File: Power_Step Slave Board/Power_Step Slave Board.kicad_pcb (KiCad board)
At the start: 2 copper layers, 69.4 x 49.1 mm, 23 parts, among them P1 CONN_01X04, P10 CONN_01X04, P11 CONN_01X02, P12 CONN_01X04, P13 CONN_01X04, P2 CONN_01X04, P3 CONN_01X02, P4 CONN_01X02, P5 CONN_01X04, P6 CONN_01X02, P7 CONN_01X04, P8 CONN_01X02, P9 CONN_01X04

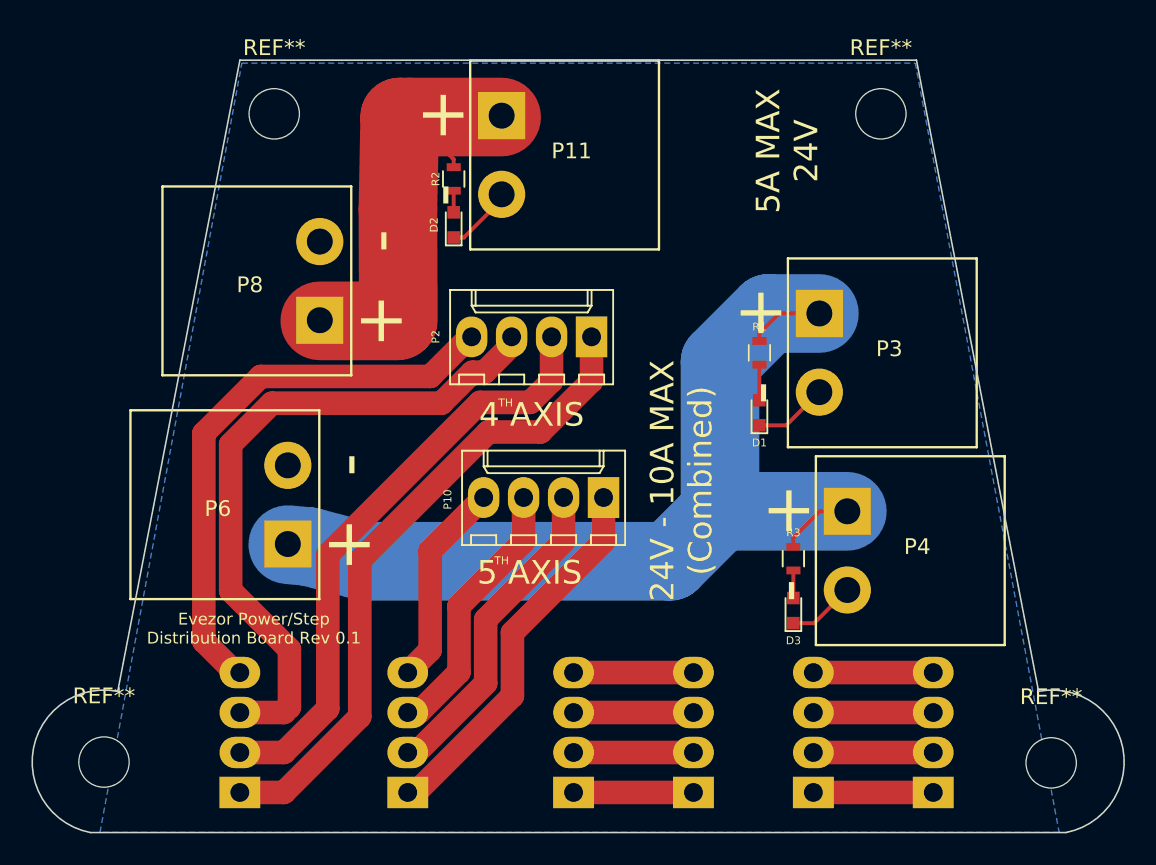
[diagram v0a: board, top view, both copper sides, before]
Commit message: more fixes
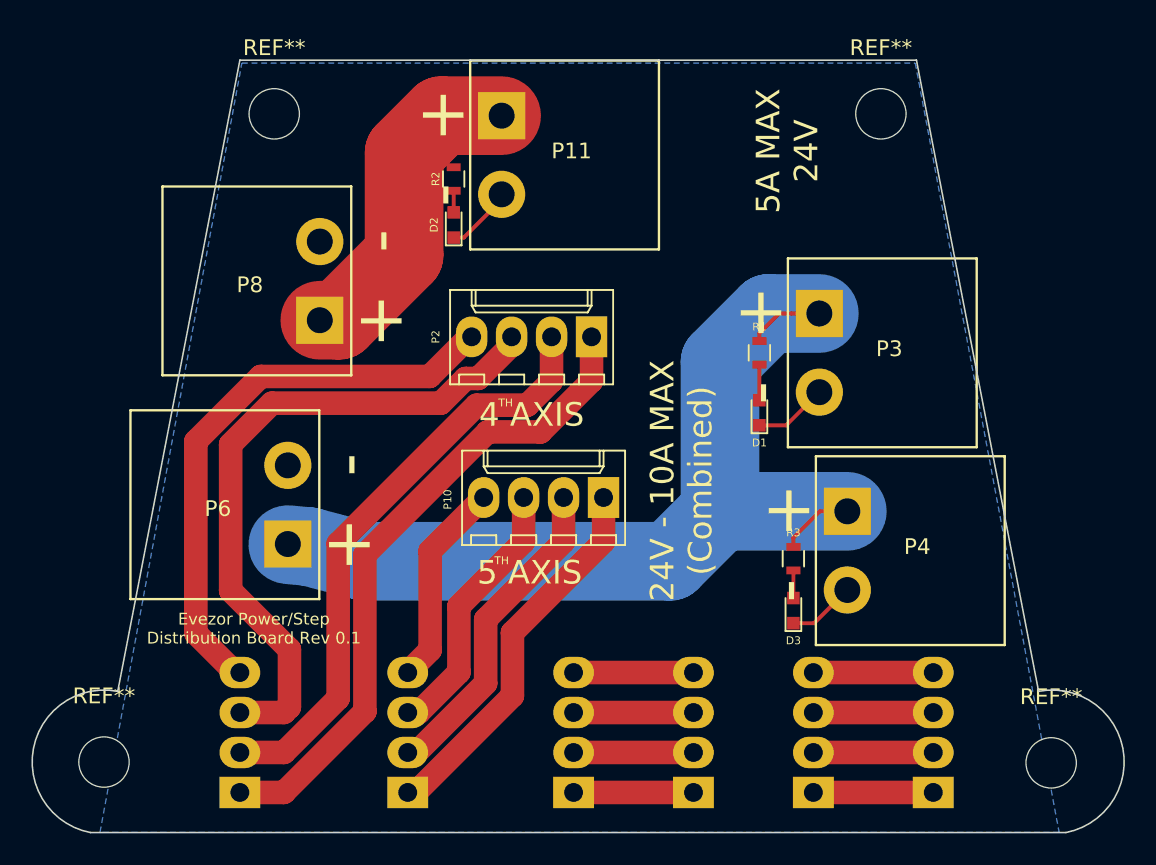
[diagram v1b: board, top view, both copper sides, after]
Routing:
- net Net-(P11-Pad2): track 29.4 -> 20.7 mm
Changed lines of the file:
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@@
     (thickness 1.6)
     (drawings 13)
-    (tracks 92)
+    (tracks 88)
     (zones 0)
     (modules 23)
@@
     (add_net "Net-(D2-Pad2)")
     (add_net "Net-(D3-Pad2)")
-    (add_net "Net-(P11-Pad2)")
     (add_net "Net-(P3-Pad2)")
   )
@@
     (uvia_dia 0.3)
     (uvia_drill 0.1)
+    (add_net "Net-(P11-Pad2)")
   )
   (module Connectors_Molex:Molex_KK-6410-04_04x2.54mm_Straight (layer F.Cu)
@@
   (segment (start 160.02 102.07) (end 160.02 99.81) (width 0.25) (layer F.Cu) (net 1))
   (segment (start 140.589 90.132) (end 140.589 88.761) (width 0.25) (layer F.Cu) (net 2))
+  (segment (start 142.748 104.0892) (end 146.1068 104.0892) (width 1.5) (layer F.Cu) (net 3))
   (segment (start 127 127) (end 129.8 127) (width 1.5) (layer F.Cu) (net 3))
-  (segment (start 129.8 127) (end 134.62 122.18) (width 1.5) (layer F.Cu) (net 3))
+  (segment (start 129.8 127) (end 134.948411 121.851589) (width 1.5) (layer F.Cu) (net 3))
+  (segment (start 134.948411 111.888789) (end 142.748 104.0892) (width 1.5) (layer F.Cu) (net 3))
+  (segment (start 134.948411 121.851589) (end 134.948411 111.888789) (width 1.5) (layer F.Cu) (net 3))
+  (segment (start 146.1068 104.0892) (end 149.352 100.844) (width 1.5) (layer F.Cu) (net 3))
   (segment (start 149.352 100.844) (end 149.352 98.044) (width 1.5) (layer F.Cu) (net 3))
-  (segment (start 134.62 122.18) (end 134.62 112.25827) (width 1.5) (layer F.Cu) (net 3))
-  (segment (start 134.62 112.25827) (end 142.78907 104.0892) (width 1.5) (layer F.Cu) (net 3))
-  (segment (start 142.78907 104.0892) (end 146.1068 104.0892) (width 1.5) (layer F.Cu) (net 3))
-  (segment (start 146.1068 104.0892) (end 149.352 100.844) (width 1.5) (layer F.Cu) (net 3))
-  (segment (start 145.4464 102.2096) (end 146.812 100.844) (width 1.5) (layer F.Cu) (net 4))
   (segment (start 127 124.46) (end 129.8 124.46) (width 1.5) (layer F.Cu) (net 4))
   (segment (start 146.812 100.844) (end 146.812 98.044) (width 1.5) (layer F.Cu) (net 4))
-  (segment (start 132.588 111.886092) (end 142.264492 102.2096) (width 1.5) (layer F.Cu) (net 4))
-  (segment (start 129.8 124.46) (end 132.588 121.672) (width 1.5) (layer F.Cu) (net 4))
-  (segment (start 132.588 121.672) (end 132.588 111.886092) (width 1.5) (layer F.Cu) (net 4))
-  (segment (start 142.264492 102.2096) (end 145.4464 102.2096) (width 1.5) (layer F.Cu) (net 4))
+  (segment (start 133.248401 111.184621) (end 142.043833 102.389189) (width 1.5) (layer F.Cu) (net 4))
+  (segment (start 133.2484 121.0116) (end 133.248401 111.184621) (width 1.5) (layer F.Cu) (net 4))
+  (segment (start 129.8 124.46) (end 133.2484 121.0116) (width 1.5) (layer F.Cu) (net 4))
+  (segment (start 142.043833 102.389189) (end 145.266811 102.389189) (width 1.5) (layer F.Cu) (net 4))
+  (segment (start 145.266811 102.389189) (end 146.812 100.844) (width 1.5) (layer F.Cu) (net 4))
+  (segment (start 129.8 121.92) (end 130.1496 121.5704) (width 1.5) (layer F.Cu) (net 5))
   (segment (start 144.272 98.56173) (end 144.272 98.044) (width 1.5) (layer F.Cu) (net 5))
-  (segment (start 141.775904 100.29401) (end 142.53972 100.29401) (width 1.5) (layer F.Cu) (net 5))
-  (segment (start 129.032 102.2604) (end 139.809514 102.2604) (width 1.5) (layer F.Cu) (net 5))
+  (segment (start 142.144552 100.689178) (end 144.272 98.56173) (width 1.5) (layer F.Cu) (net 5))
+  (segment (start 141.339666 100.689178) (end 142.144552 100.689178) (width 1.5) (layer F.Cu) (net 5))
   (segment (start 126.414011 104.878389) (end 129.032 102.2604) (width 1.5) (layer F.Cu) (net 5))
   (segment (start 126.414011 114.171211) (end 126.414011 104.878389) (width 1.5) (layer F.Cu) (net 5))
+  (segment (start 139.768444 102.2604) (end 141.339666 100.689178) (width 1.5) (layer F.Cu) (net 5))
+  (segment (start 129.032 102.2604) (end 139.768444 102.2604) (width 1.5) (layer F.Cu) (net 5))
   (segment (start 130.1496 117.9068) (end 126.414011 114.171211) (width 1.5) (layer F.Cu) (net 5))
+  (segment (start 127 121.92) (end 129.8 121.92) (width 1.5) (layer F.Cu) (net 5))
   (segment (start 130.1496 121.5704) (end 130.1496 117.9068) (width 1.5) (layer F.Cu) (net 5))
-  (segment (start 127 121.92) (end 129.8 121.92) (width 1.5) (layer F.Cu) (net 5))
-  (segment (start 129.8 121.92) (end 130.1496 121.5704) (width 1.5) (layer F.Cu) (net 5))
-  (segment (start 142.53972 100.29401) (end 144.272 98.56173) (width 1.5) (layer F.Cu) (net 5))
-  (segment (start 139.809514 102.2604) (end 141.775904 100.29401) (width 1.5) (layer F.Cu) (net 5))
-  (segment (start 128.327833 100.560389) (end 124.714 104.174222) (width 1.5) (layer F.Cu) (net 6))
-  (segment (start 139.105347 100.560389) (end 128.327833 100.560389) (width 1.5) (layer F.Cu) (net 6))
-  (segment (start 141.732 98.044) (end 141.621736 98.044) (width 1.5) (layer F.Cu) (net 6))
-  (segment (start 141.621736 98.044) (end 139.105347 100.560389) (width 1.5) (layer F.Cu) (net 6))
-  (segment (start 124.714 104.174222) (end 124.714 117.394) (width 1.5) (layer F.Cu) (net 6))
-  (segment (start 124.714 117.394) (end 126.7 119.38) (width 1.5) (layer F.Cu) (net 6))
+  (segment (start 139.064277 100.560389) (end 128.327833 100.560389) (width 1.5) (layer F.Cu) (net 6))
+  (segment (start 141.732 98.044) (end 141.580666 98.044) (width 1.5) (layer F.Cu) (net 6))
+  (segment (start 124.2 104.688222) (end 124.2 116.88) (width 1.5) (layer F.Cu) (net 6))
+  (segment (start 124.2 116.88) (end 126.7 119.38) (width 1.5) (layer F.Cu) (net 6))
+  (segment (start 128.327833 100.560389) (end 124.2 104.688222) (width 1.5) (layer F.Cu) (net 6))
+  (segment (start 141.580666 98.044) (end 139.064277 100.560389) (width 1.5) (layer F.Cu) (net 6))
   (segment (start 126.7 119.38) (end 127 119.38) (width 1.5) (layer F.Cu) (net 6))
   (segment (start 162.179 111.391) (end 162.179 110.812) (width 0.25) (layer F.Cu) (net 7))
@@
   (segment (start 148.209 121.92) (end 155.829 121.92) (width 1.5) (layer F.Cu) (net 10))
   (segment (start 155.829 119.38) (end 148.209 119.38) (width 1.5) (layer F.Cu) (net 11))
-  (segment (start 140.589 87.261) (end 140.589 86.761) (width 0.25) (layer F.Cu) (net 12))
-  (segment (start 140.589 86.761) (end 137.902 84.074) (width 0.25) (layer F.Cu) (net 12))
-  (segment (start 137.902 84.074) (end 137.16 84.074) (width 0.25) (layer F.Cu) (net 12))
-  (segment (start 132.08 97.028) (end 137.033 97.028) (width 5) (layer F.Cu) (net 12))
-  (segment (start 137.16 84.074) (end 137.795 84.074) (width 5) (layer F.Cu) (net 12))
-  (segment (start 137.795 84.074) (end 143.637 84.074) (width 5) (layer F.Cu) (net 12))
-  (segment (start 137.045 89.928) (end 137.16 84.074) (width 5) (layer F.Cu) (net 12))
-  (segment (start 137.073 96.988) (end 137.045 89.928) (width 5) (layer F.Cu) (net 12))
-  (segment (start 137.033 97.028) (end 137.073 96.988) (width 0.25) (layer F.Cu) (net 12))
+  (segment (start 132.08 96.988) (end 133.296002 96.988) (width 5) (layer F.Cu) (net 12))
+  (segment (start 133.296002 96.988) (end 137.438999 92.845003) (width 5) (layer F.Cu) (net 12))
+  (segment (start 137.438999 92.845003) (end 137.438999 86.350999) (width 5) (layer F.Cu) (net 12))
+  (segment (start 137.438999 86.350999) (end 139.802998 83.987) (width 5) (layer F.Cu) (net 12))
+  (segment (start 139.802998 83.987) (end 143.637 83.987) (width 5) (layer F.Cu) (net 12))
   (segment (start 138.18573 127) (end 144.3228 120.86293) (width 1.5) (layer F.Cu) (net 13))
   (segment (start 150.114 111.0548) (end 150.114 108.2548) (width 1.5) (layer F.Cu) (net 13))

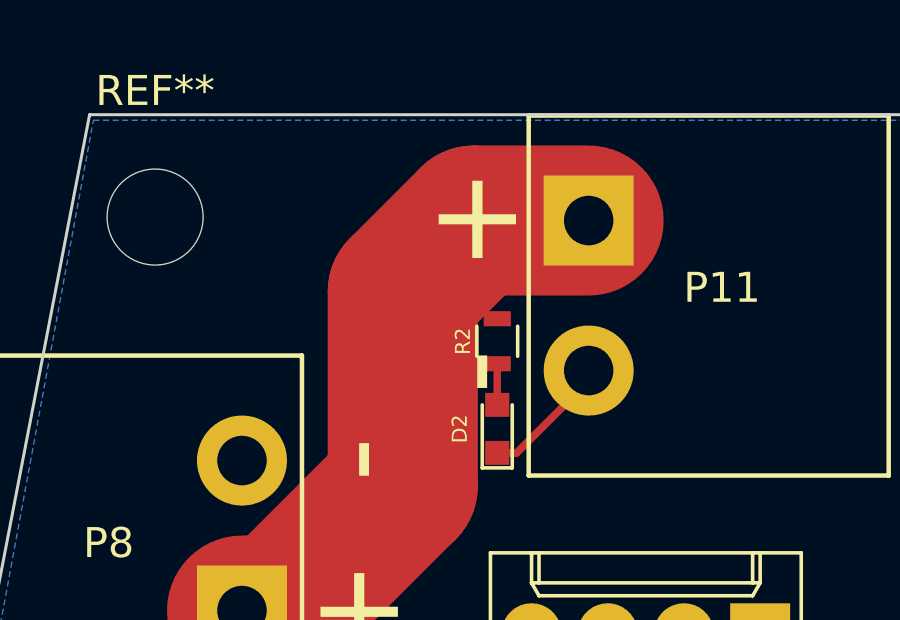
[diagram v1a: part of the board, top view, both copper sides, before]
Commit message: suggested changes
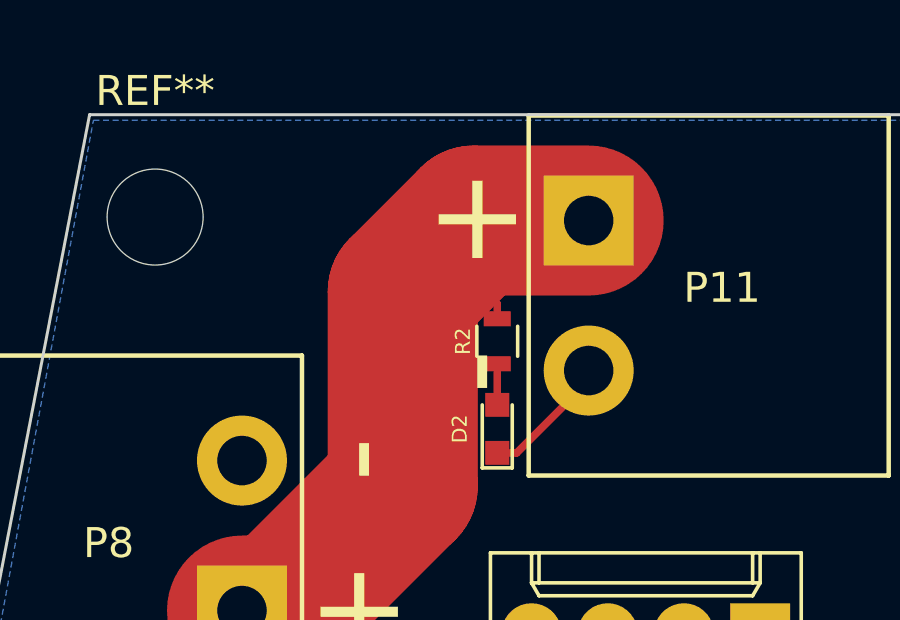
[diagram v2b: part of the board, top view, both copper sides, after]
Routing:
- net Net-(P11-Pad2): track 20.7 -> 24.6 mm
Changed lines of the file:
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@@
     (links 32)
     (no_connects 0)
-    (area 113.74941 80.211999 183.252791 129.598203)
+    (area 113.74941 80.408997 183.252791 129.598203)
     (thickness 1.6)
     (drawings 13)
-    (tracks 88)
+    (tracks 91)
     (zones 0)
     (modules 23)
@@
     (add_net "Net-(D2-Pad2)")
     (add_net "Net-(D3-Pad2)")
+    (add_net "Net-(P11-Pad2)")
     (add_net "Net-(P3-Pad2)")
   )
@@
     (uvia_dia 0.3)
     (uvia_drill 0.1)
-    (add_net "Net-(P11-Pad2)")
   )
   (module Connectors_Molex:Molex_KK-6410-04_04x2.54mm_Straight (layer F.Cu)
@@
   (segment (start 148.209 121.92) (end 155.829 121.92) (width 1.5) (layer F.Cu) (net 10))
   (segment (start 155.829 119.38) (end 148.209 119.38) (width 1.5) (layer F.Cu) (net 11))
+  (segment (start 140.589 87.261) (end 140.589 86.761) (width 0.25) (layer F.Cu) (net 12))
+  (segment (start 140.589 86.761) (end 140.178999 86.350999) (width 0.25) (layer F.Cu) (net 12))
+  (segment (start 140.178999 86.350999) (end 137.438999 86.350999) (width 0.25) (layer F.Cu) (net 12))
   (segment (start 132.08 96.988) (end 133.296002 96.988) (width 5) (layer F.Cu) (net 12))
   (segment (start 133.296002 96.988) (end 137.438999 92.845003) (width 5) (layer F.Cu) (net 12))
